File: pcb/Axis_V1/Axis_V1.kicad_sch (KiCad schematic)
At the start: 33 parts, among them J1 Screw_Terminal_01x03, J10 BOILER_3v3, J11 3WAY_L, J2 Screw_Terminal_01x03, J3 BREW_SW, J4 STEAM_SW, J5 AC_L, J6 AC_N, J7 BOILER_GND, J9 PUMP_L, Q1 BC547, Q2 BT136-500, Q3 BT136-500, U1 Pico, U2 ADS1115IDGS, U3 MAX31855KASA

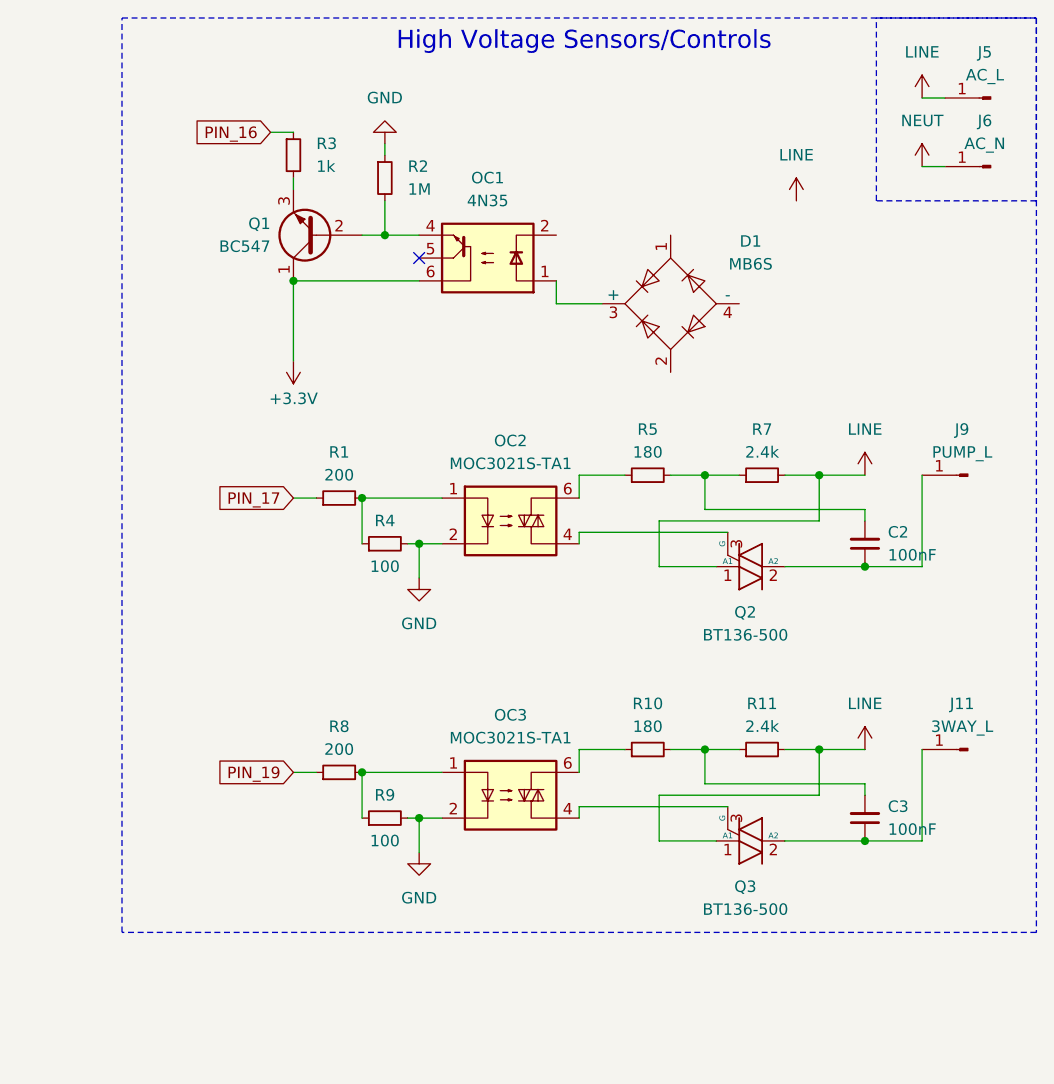
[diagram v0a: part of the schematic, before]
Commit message: PCB Updates
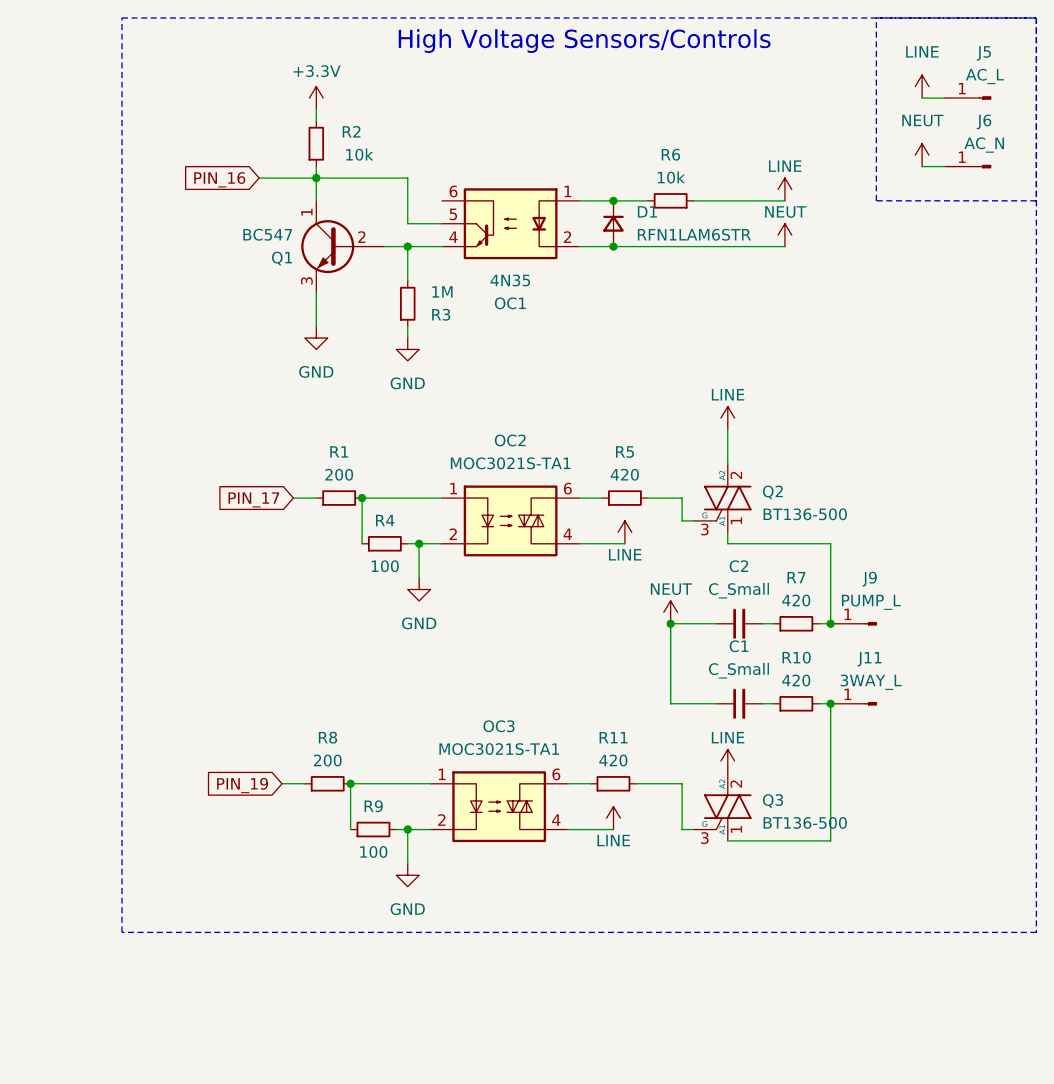
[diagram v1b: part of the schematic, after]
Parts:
- removed C3: 100nF, Capacitor_SMD:C_0402_1005Metric, symbol Device:C_Small
- removed D1: MB6S, Package_TO_SOT_SMD:TO-269AA, symbol Diode_Bridge:MB6S
- added C1: C_Small, Resistor_SMD:R_2512_6332Metric, symbol Device:C_Small
- added D1: RFN1LAM6STR, Diode_SMD:D_SOD-128, symbol Device:D_Small
- added R6: 10k, Resistor_SMD:R_2512_6332Metric, symbol Device:R_Small
- C2: value 100nF -> C_Small; footprint Capacitor_SMD:C_0402_1005Metric -> Resistor_SMD:R_2512_6332Metric
- OC1, OC2, OC3: footprint DIP:SMDIP-6_W7.62mm -> Package_DIP:SMDIP-6_W7.62mm
- R10, R5: value 180 -> 420
- R11, R7: value 2.4k -> 420
- R2: value 1M -> 10k
- R3: value 1k -> 1M
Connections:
- net +3.3V: now also R2.2; no longer OC1.6, Q1.1 (C)
- net GND: now also Q1.3 (E), R3.1; no longer R2.1
- net LINE: now also OC2.4, OC3.4, Q2.2 (A2), Q3.2 (A2), R6.1; no longer Q2.1 (A1), Q3.1 (A1), R11.2, R7.2
- net NEUT: now also C2.1, OC1.2, C1.1, D1.2 (A)
- net PIN_16: now also OC1.5, Q1.1 (C), R2.1; no longer R3.1
- net at C2.2, R7.1: no longer R5.2
- net at R10.2: now also J11.1 (Pin_1), Q3.1 (A1); no longer R11.1
- net at Q2.3 (G): now also R5.2; no longer OC2.4
- net at R10.1: now also C1.2; no longer OC3.6
- net at OC1.1: now also D1.1 (K), R6.2
- net at OC1.4, Q1.2 (B): now also R3.2; no longer R2.2
- net at Q3.3 (G): now also R11.2; no longer OC3.4
- new net: J9.1 (Pin_1), Q2.1 (A1), R7.2
- new net: OC3.6, R11.1
- no-connect marks 22 -> 21
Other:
- moved on the sheet: J11, J9, OC1, OC3, Q2, R8, R9
